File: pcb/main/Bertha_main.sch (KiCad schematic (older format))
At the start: 85 parts, among them J1 RJ12, J12 AudioJack3_SwitchTR, J2 Conn_Coaxial_Power, J3 Conn_02x03_Odd_Even, J4 RJ12, J5 AudioJack3_SwitchTR, J6 SJ, J7 Conn_01x01, J8 Conn_01x01, Q1 ZXMS6004, Q2 ZXMS6004, Q3 IPB80N03S4L-03, Q5 ZXMS6004, Q6 ZXMS6004, Q7 ZXMS6004, U1 DS18B20, U2 ATMEGA32U4-AU, X1 MINI-USB-SCHIELD-32005-201, Y1 Crystal

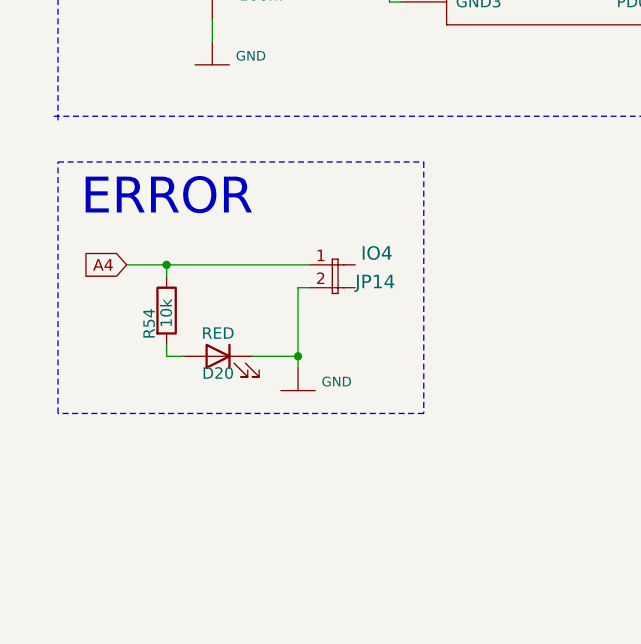
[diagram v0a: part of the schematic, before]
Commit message: New place for ERROR and add transistor for LED-strip (issue #37)
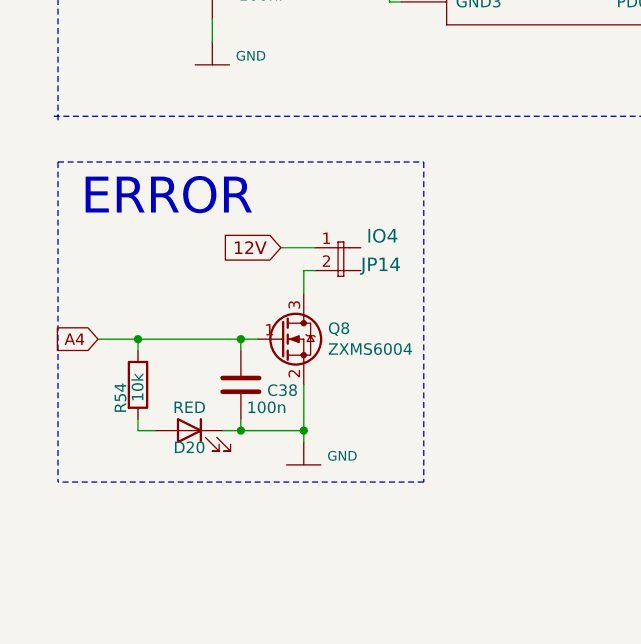
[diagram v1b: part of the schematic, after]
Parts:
- added C38: 100n, Capacitor_SMD:C_0805_2012Metric_Pad1.15x1.40mm_HandSolder, symbol Device:C
- added Q8: ZXMS6004, Package_TO_SOT_SMD:SOT-23, symbol ZXMS6004:ZXMS6004
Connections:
- net 12V: now also JP14.1
- net A4: now also C38.1, Q8.1 (G); no longer JP14.1
- net at D20.1 (K): now also C38.2, Q8.2 (S); no longer JP14.2
- new net: JP14.2, Q8.3 (D)
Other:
- moved on the sheet: D20, JP14, R54
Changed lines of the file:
@@
 L Bertha_main-eagle-import:JP1E JP?
 U 1 1 5F6B070F
-P 2075 8200
+P 2100 8125
 AR Path="/5E0D793B/5F6B070F" Ref="JP?"  Part="1"
 AR Path="/5F6B070F" Ref="JP14"  Part="1"
-F 0 "JP14" V 2150 8300 59  0000 L CNN
-F 1 "IO4" V 2025 8325 59  0000 L CNN
-F 2 "Connector_Molex:Molex_KK-254_AE-6410-02A_1x02_P2.54mm_Vertical" H 2075 8200 50  0001 C CNN
-F 3 "" H 2075 8200 50  0001 C CNN
-	1    2075 8200
+F 0 "JP14" V 2175 8225 59  0000 L CNN
+F 1 "IO4" V 2050 8250 59  0000 L CNN
+F 2 "Connector_Molex:Molex_KK-254_AE-6410-02A_1x02_P2.54mm_Vertical" H 2100 8125 50  0001 C CNN
+F 3 "" H 2100 8125 50  0001 C CNN
+	1    2100 8125
 	0    1    1    0
 $EndComp
@@
 L Device:LED D?
 U 1 1 5F6B0F69
-P 1575 8600
+P 1450 8925
 AR Path="/5E0005EE/5F6B0F69" Ref="D?"  Part="1"
 AR Path="/5F6B0F69" Ref="D20"  Part="1"
-F 0 "D20" H 1575 8525 50  0000 C CNN
-F 1 "RED" H 1575 8700 50  0000 C CNN
-F 2 "LED_SMD:LED_0805_2012Metric_Pad1.15x1.40mm_HandSolder" H 1575 8600 50  0001 C CNN
-F 3 "~" H 1575 8600 50  0001 C CNN
-	1    1575 8600
+F 0 "D20" H 1450 8850 50  0000 C CNN
+F 1 "RED" H 1450 9025 50  0000 C CNN
+F 2 "LED_SMD:LED_0805_2012Metric_Pad1.15x1.40mm_HandSolder" H 1450 8925 50  0001 C CNN
+F 3 "~" H 1450 8925 50  0001 C CNN
+	1    1450 8925
 	-1   0    0    -1
 $EndComp
@@
 L Device:R R?
 U 1 1 5F6B1D75
-P 1350 8400
+P 1225 8725
 AR Path="/5E0D7B15/5F6B1D75" Ref="R?"  Part="1"
 AR Path="/5F6B1D75" Ref="R54"  Part="1"
-F 0 "R54" V 1275 8275 50  0000 L CNN
-F 1 "10k" V 1350 8325 50  0000 L CNN
-F 2 "Resistor_SMD:R_0805_2012Metric_Pad1.15x1.40mm_HandSolder" V 1280 8400 50  0001 C CNN
-F 3 "~" H 1350 8400 50  0001 C CNN
-	1    1350 8400
+F 0 "R54" V 1150 8600 50  0000 L CNN
+F 1 "10k" V 1225 8650 50  0000 L CNN
+F 2 "Resistor_SMD:R_0805_2012Metric_Pad1.15x1.40mm_HandSolder" V 1155 8725 50  0001 C CNN
+F 3 "~" H 1225 8725 50  0001 C CNN
+	1    1225 8725
 	1    0    0    -1
 $EndComp
 Text GLabel 4425 4250 2    50   Input ~ 0
 A4
-Text GLabel 1175 8200 0    50   Input ~ 0
+Text GLabel 1050 8525 0    50   Input ~ 0
 A4
 Wire Wire Line
-	1975 8200 1350 8200
+	1225 8575 1225 8525
 Wire Wire Line
-	1350 8250 1350 8200
-Connection ~ 1350 8200
+	1225 8525 1050 8525
 Wire Wire Line
-	1350 8200 1175 8200
+	1300 8925 1225 8925
 Wire Wire Line
-	1425 8600 1350 8600
-Wire Wire Line
-	1350 8600 1350 8550
+	1225 8925 1225 8875
 $Comp
 L Bertha_main-eagle-import:GND #0102
 U 1 1 5F75493A
-P 1925 8750
-F 0 "#0102" H 1975 8800 50  0001 C CNN
-F 1 "GND" H 2028 8788 42  0000 L CNN
-F 2 "" H 1925 8750 50  0001 C CNN
-F 3 "" H 1925 8750 50  0001 C CNN
-	1    1925 8750
+P 1950 9075
+F 0 "#0102" H 2000 9125 50  0001 C CNN
+F 1 "GND" H 2053 9113 42  0000 L CNN
+F 2 "" H 1950 9075 50  0001 C CNN
+F 3 "" H 1950 9075 50  0001 C CNN
+	1    1950 9075
 	1    0    0    -1
 $EndComp
 Wire Wire Line
-	1975 8300 1925 8300
+	2000 8225 1950 8225
 Wire Wire Line
-	1925 8300 1925 8600
-Wire Wire Line
-	1725 8600 1925 8600
-Connection ~ 1925 8600
-Wire Wire Line
-	1925 8600 1925 8650
+	1600 8925 1675 8925
 Wire Notes Line
 	875  7750 2475 7750
 Wire Notes Line
-	2475 7750 2475 8850
+	2475 9150 875  9150
+$Comp
+L ZXMS6004:ZXMS6004 Q8
+U 1 1 5F4A21DB
+P 1950 8525
+F 0 "Q8" H 2056 8571 50  0000 L CNN
+F 1 "ZXMS6004" H 2056 8480 50  0000 L CNN
+F 2 "Package_TO_SOT_SMD:SOT-23" H 2050 8450 50  0001 L CIN
+F 3 "https://www.diodes.com/assets/Datasheets/ZXMS6004FF.pdf" H 2050 8600 50  0001 L CNN
+	1    1950 8525
+	1    0    0    -1
+$EndComp
+$Comp
+L Device:C C?
+U 1 1 5F4A3E1A
+P 1675 8725
+AR Path="/5E02557B/5F4A3E1A" Ref="C?"  Part="1"
+AR Path="/5F4A3E1A" Ref="C38"  Part="1"
+F 0 "C38" H 1425 8700 50  0000 L CNN
+F 1 "100n" H 1475 8625 50  0000 L CNN
+F 2 "Capacitor_SMD:C_0805_2012Metric_Pad1.15x1.40mm_HandSolder" H 1713 8575 50  0001 C CNN
+F 3 "~" H 1675 8725 50  0001 C CNN
+	1    1675 8725
+	-1   0    0    -1
+$EndComp
+Text GLabel 1850 8125 0    55   Input ~ 0
+12V
+Wire Wire Line
+	1750 8525 1675 8525
+Wire Wire Line
+	1675 8525 1675 8575
+Wire Wire Line
+	1675 8525 1225 8525
+Connection ~ 1675 8525
+Connection ~ 1225 8525
+Wire Wire Line
+	1675 8875 1675 8925
+Connection ~ 1675 8925
+Wire Wire Line
+	1950 8725 1950 8925
+Wire Wire Line
+	1675 8925 1950 8925
+Connection ~ 1950 8925
+Wire Wire Line
+	1950 8925 1950 8975
+Wire Wire Line
+	2000 8125 1850 8125
+Wire Wire Line
+	1950 8225 1950 8325
 Wire Notes Line
-	2475 8850 875  8850
+	2475 7750 2475 9150
 Wire Notes Line
-	875  8850 875  7750
+	875  7750 875  9150
 $EndSCHEMATC
